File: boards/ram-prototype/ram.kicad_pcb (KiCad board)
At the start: 4 copper layers, 158 x 90 mm, 391 parts, among them J1 PinHeader_1x16_P2.54mm_Vertic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, U1 DSBGA\-5_NumericPads, U10 DSBGA\-5_NumericPads, U100 DSBGA\-5_NumericPads, U101 DSBGA\-5_NumericPads, U102 DSBGA\-5_NumericPads, U103 DSBGA\-5_NumericPads, U104 DSBGA\-5_NumericPads, U105 DSBGA\-5_NumericPads, U106 DSBGA\-5_NumericPads, U107 DSBGA\-5_NumericPads, U108 DSBGA\-5_NumericPads, U109 DSBGA\-5_NumericPads, U11 DSBGA\-5_NumericPads, U110 DSBGA\-5_NumericPads, U111 DSBGA\-5_NumericPads, U112 DSBGA\-5_NumericPads, U113 DSBGA\-5_NumericPads, U114 DSBGA\-5_NumericPads, U115 DSBGA\-5_NumericPads, U116 DSBGA\-5_NumericPads, U117 DSBGA\-5_NumericPads, U118 DSBGA\-5_NumericPads, U119 DSBGA\-5_NumericPads, U12 DSBGA\-5_NumericPads, U120 DSBGA\-5_NumericPads, U121 DSBGA\-5_NumericPads, U122 DSBGA\-5_NumericPads, U123 DSBGA\-5_NumericPads, U124 DSBGA\-5_NumericPads, U125 DSBGA\-5_NumericPads, U126 DSBGA\-5_NumericPads, U127 DSBGA\-5_NumericPads, U128 DSBGA\-5_NumericPads, U129 DSBGA\-5_NumericPads, U13 DSBGA\-5_NumericPads, U130 DSBGA\-5_NumericPads, U131 DSBGA\-5_NumericPads, U132 DSBGA\-5_NumericPads, U133 DSBGA\-5_NumericPads, U134 DSBGA\-5_NumericPads, U135 DSBGA\-5_NumericPads, U136 DSBGA\-5_NumericPads, U137 DSBGA\-5_NumericPads, U138 DSBGA\-5_NumericPads, U139 DSBGA\-5_NumericPads, U14 DSBGA\-5_NumericPads, U140 DSBGA\-5_NumericPads, U141 DSBGA\-5_NumericPads, U142 DSBGA\-5_NumericPads, U143 DSBGA\-5_NumericPads, U144 DSBGA\-5_NumericPads, U145 DSBGA\-5_NumericPads, U146 DSBGA\-5_NumericPads, U147 DSBGA\-5_NumericPads, U148 DSBGA\-5_NumericPads, U149 DSBGA\-5_NumericPads, U15 DSBGA\-5_NumericPads, U150 DSBGA\-5_NumericPads, U151 DSBGA\-5_NumericPads, U152 DSBGA\-5_NumericPads, U153 DSBGA\-5_NumericPads, U154 DSBGA\-5_NumericPads, U155 DSBGA\-5_NumericPads, U156 DSBGA\-5_NumericPads, U157 DSBGA\-5_NumericPads, U158 DSBGA\-5_NumericPads, U16 DSBGA\-5_NumericPads, U17 DSBGA\-5_NumericPads, U18 DSBGA\-5_NumericPads, U19 DSBGA\-5_NumericPads, U2 DSBGA\-5_NumericPads, U20 DSBGA\-5_NumericPads, U21 DSBGA\-5_NumericPads, U22 DSBGA\-5_NumericPads, U23 DSBGA\-8_NumericPads, U24 DSBGA\-8_NumericPads, U25 DSBGA\-8_NumericPads, U26 DSBGA\-8_NumericPads, U27 DSBGA\-8_NumericPads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

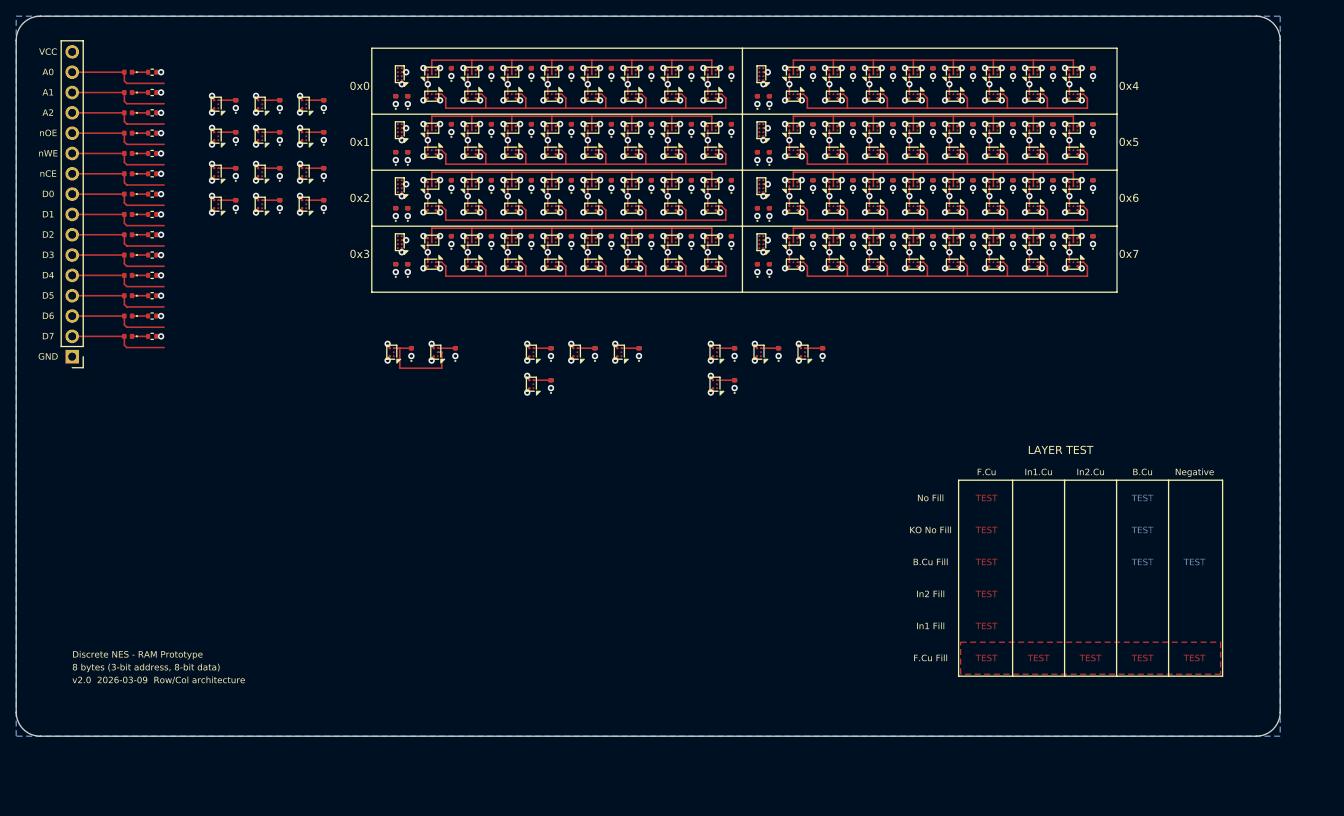
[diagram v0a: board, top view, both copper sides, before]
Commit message: Change layout
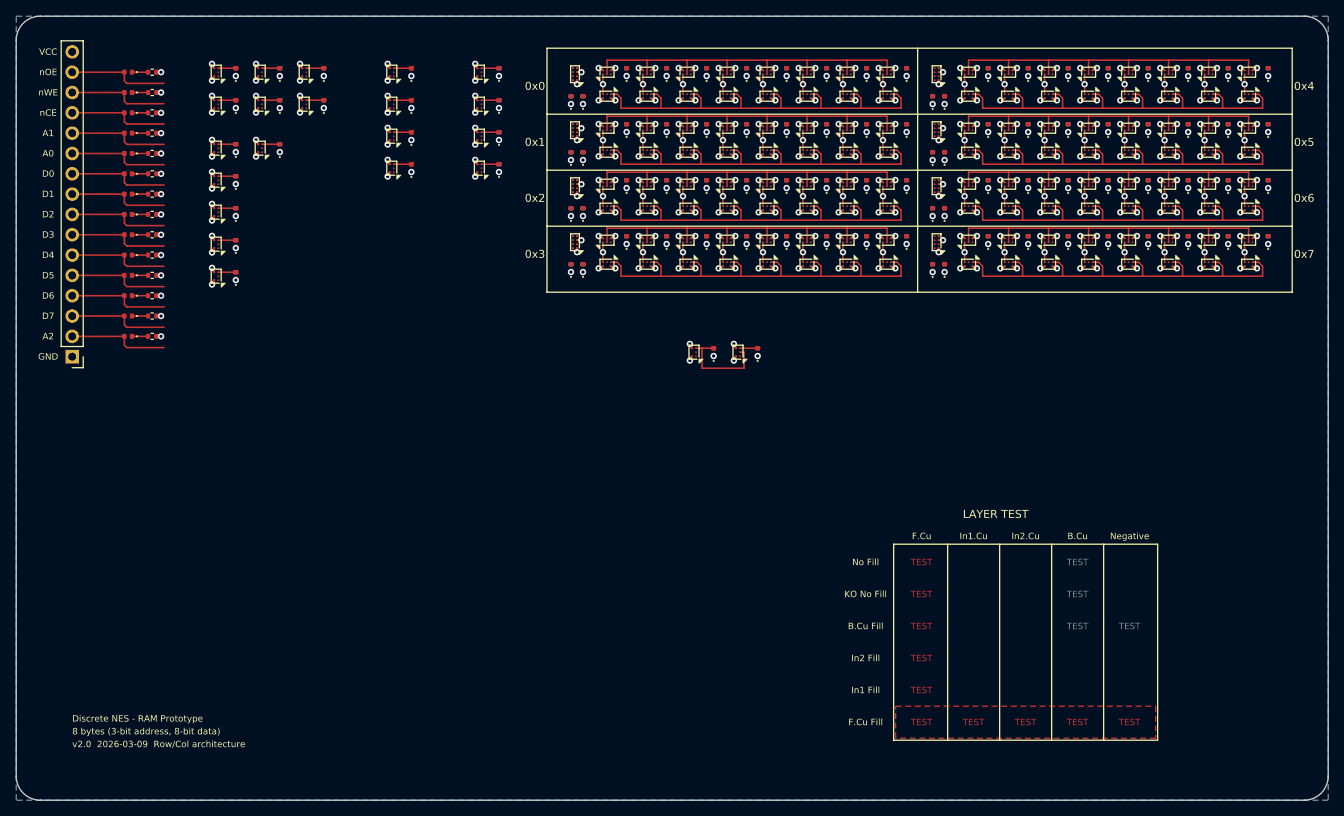
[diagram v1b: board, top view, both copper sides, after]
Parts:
- moved D35 48.6 mm to (73.3, 28.0)
- moved R35 48.6 mm to (73.3, 28.0)
- moved U21 48.6 mm to (70.9, 28.0)
- moved D34 46.7 mm to (73.3, 24.0)
- moved R34 46.7 mm to (73.3, 24.0)
- moved U20 46.7 mm to (70.9, 24.0)
- moved D33 45.7 mm to (73.3, 20.0)
- moved R33 45.7 mm to (73.3, 20.0)
- moved U19 45.7 mm to (70.9, 20.0)
- moved D36 40.0 mm to (73.3, 32.0)
- moved R36 40.0 mm to (73.3, 32.0)
- moved U22 40.0 mm to (70.9, 32.0)
- moved D31 39.2 mm to (62.4, 28.0)
- moved R31 39.2 mm to (62.4, 28.0)
- moved U17 39.2 mm to (60.0, 28.0)
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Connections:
- D1 pad 2: /Address Decoder/A0 -> /Control Logic/nOE
- D10 pad 2: /D3 -> /D4
- D11 pad 2: /D4 -> /D5
- D12 pad 2: /D5 -> /D6
- D13 pad 2: /D6 -> /D7
- D14 pad 2: /D7 -> /Column Select/A2
- D2 pad 2: /Address Decoder/A1 -> /Control Logic/nWE
- D3 pad 2: /Column Select/A2 -> /Control Logic/nCE
- D4 pad 2: /Control Logic/nOE -> /Address Decoder/A1
- D5 pad 2: /Control Logic/nWE -> /Address Decoder/A0
- D6 pad 2: /Control Logic/nCE -> /D0
- D7 pad 2: /D0 -> /D1
- D8 pad 2: /D1 -> /D2
- D9 pad 2: /D2 -> /D3
- J1 pad 10: /Control Logic/nCE -> /D0
- J1 pad 11: /Control Logic/nWE -> /Address Decoder/A0
- J1 pad 12: /Control Logic/nOE -> /Address Decoder/A1
- J1 pad 13: /Column Select/A2 -> /Control Logic/nCE
- J1 pad 14: /Address Decoder/A1 -> /Control Logic/nWE
- J1 pad 15: /Address Decoder/A0 -> /Control Logic/nOE
- J1 pad 2: /D7 -> /Column Select/A2
- J1 pad 3: /D6 -> /D7
- J1 pad 4: /D5 -> /D6
- J1 pad 5: /D4 -> /D5
- J1 pad 6: /D3 -> /D4
- J1 pad 7: /D2 -> /D3
- J1 pad 8: /D1 -> /D2
- J1 pad 9: /D0 -> /D1
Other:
- board size 158 x 90 mm -> 164 x 98 mm
